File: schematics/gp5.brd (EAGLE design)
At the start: 40 x 30 mm, 11 parts, among them IC1 317T, IC2 317EMP, IC3 TLE5205-2S

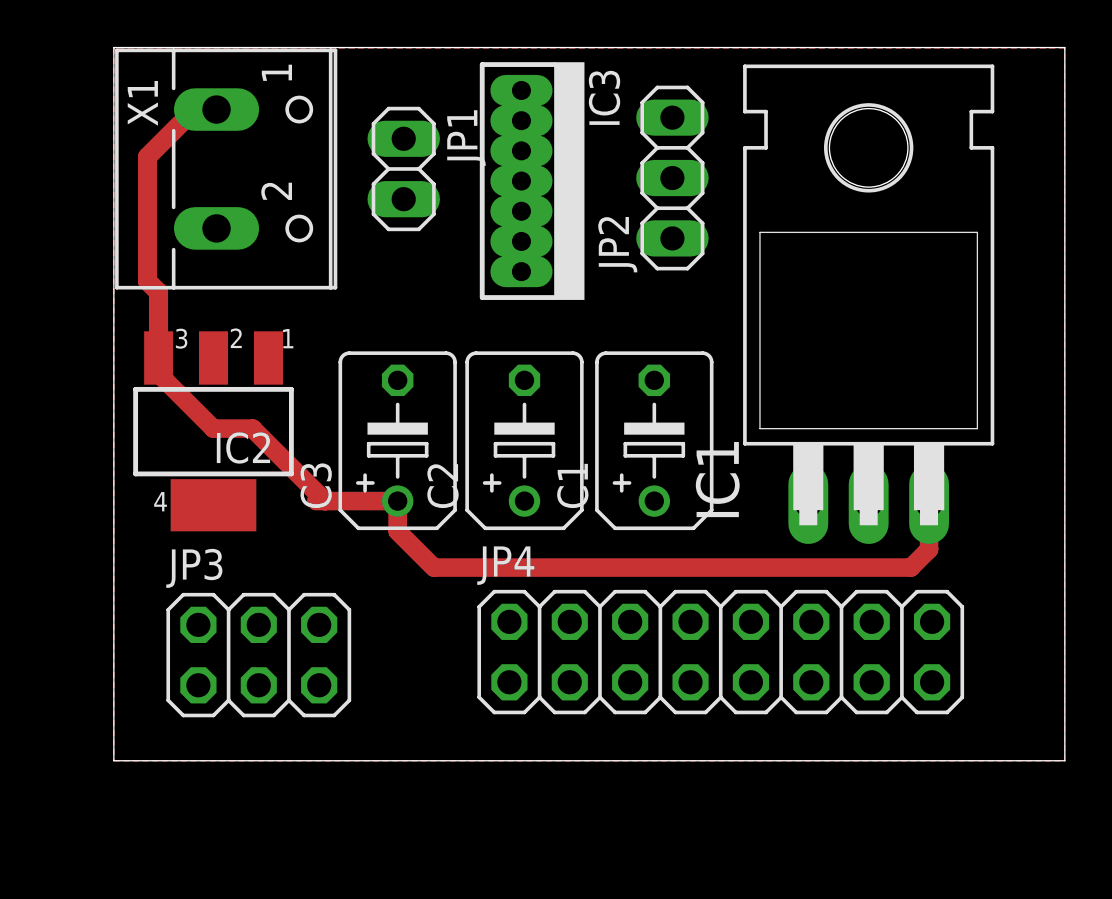
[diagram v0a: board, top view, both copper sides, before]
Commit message: finalised schematic files
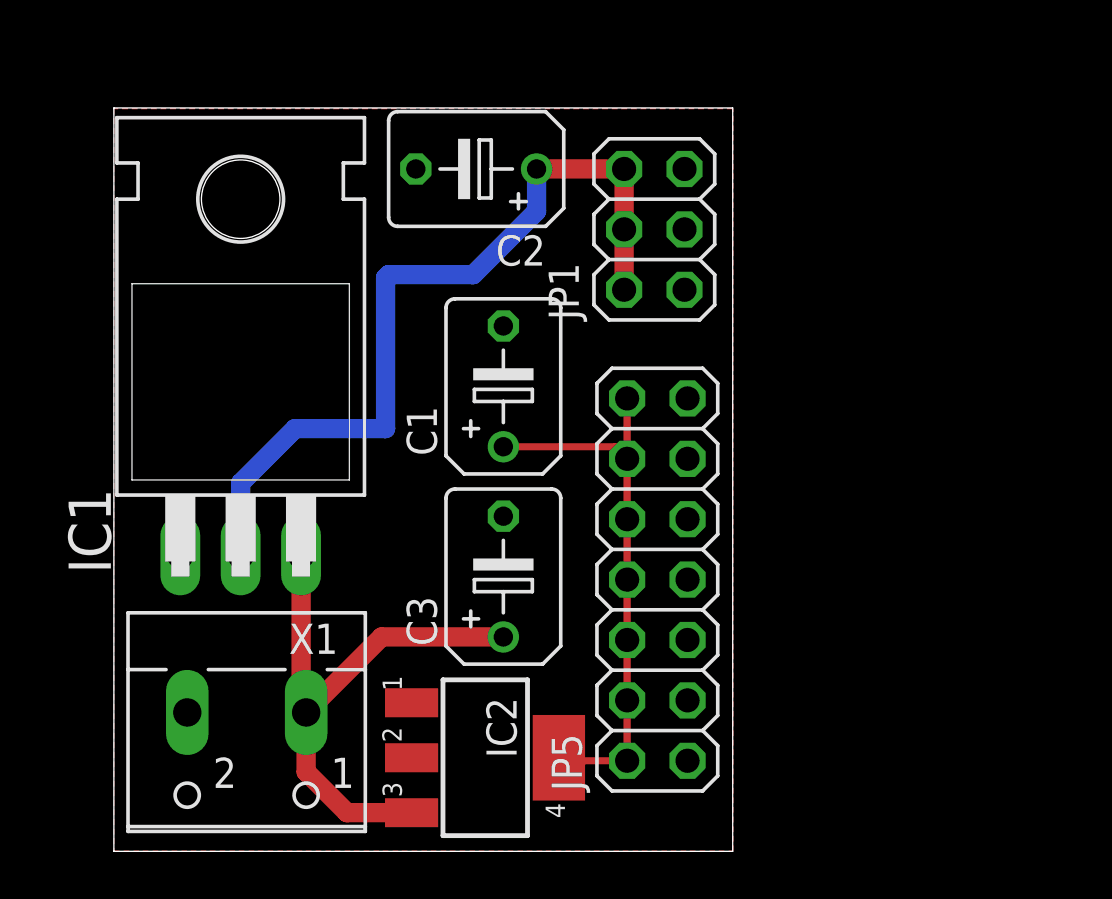
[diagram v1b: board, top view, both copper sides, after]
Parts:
- removed IC3: TLE5205-2S, infineon:P-TO220-7-12
- removed JP2: (no value), pinhead:1X03
- removed JP3: (no value), pinhead:2X03
- removed JP4: (no value), pinhead:2X08
- added JP5: (no value), pinhead:2X07
- JP1: device pinhead:1X02 -> pinhead:2X03
- moved IC1 26.5 mm to (5.33, 18.8)
- moved X1 24.1 mm to (5.59, 0.76), turned to 180 degrees
- moved IC2 17.9 mm to (15.6, 0.13), turned to 270 degrees
- moved C2 11.6 mm to (15.2, 24.9), turned to 180 degrees
- moved JP1 10.8 mm to (22.7, 22.4), turned to 90 degrees
- moved C3 7.24 mm to (16.4, 7.75)
- moved C1 6.75 mm to (16.4, 15.7)
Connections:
- removed net MOTOR_OUT1: IC3.1, JP1.1
- removed net N$2: IC3.7, JP1.2
- removed net N$3: IC3.2, JP2.3
- removed net N$4: IC3.3, JP2.2
- removed net N$5: IC3.5, JP2.1
- net +3.3V: now also JP5.10, JP5.12, JP5.14, JP5.2, JP5.4, JP5.6, JP5.8; no longer JP3.2, JP3.4, JP3.6
- net +5V_R: now also JP1.2, JP1.4, JP1.6; no longer IC3.6, JP4.10, JP4.12, JP4.14, JP4.16, JP4.2, JP4.4, JP4.6, JP4.8
- net GND: now also JP1.1, JP1.3, JP1.5, JP5.1, JP5.11, JP5.13, JP5.3, JP5.5, JP5.7, JP5.9; no longer IC3.4, JP3.1, JP3.3, JP3.5, JP4.1, JP4.11, JP4.13, JP4.15, JP4.3, JP4.5, JP4.7, JP4.9
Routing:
- net +5V_R: track 0.00 -> 34.5 mm
- net 8.4V: track 52.2 -> 23.9 mm
- net +3.3V: track 0.00 -> 23.6 mm
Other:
- board size 40 x 30 mm -> 26 x 31.3 mm
